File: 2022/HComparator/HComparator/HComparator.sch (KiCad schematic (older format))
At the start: 0 parts

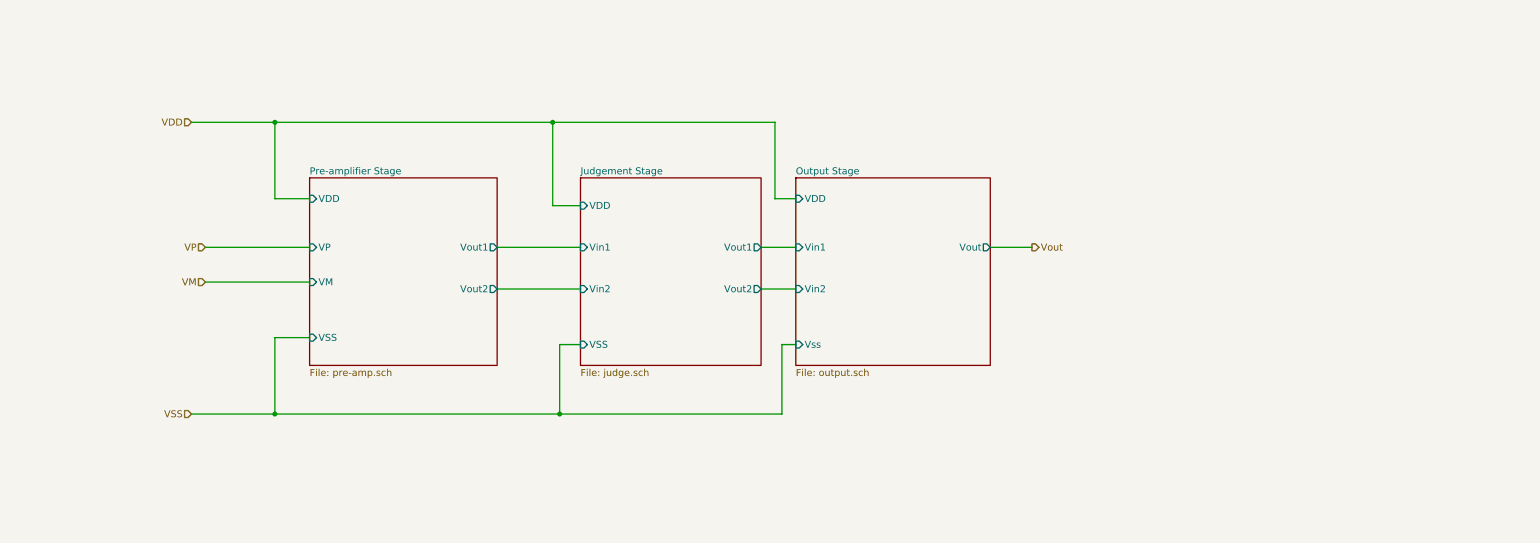
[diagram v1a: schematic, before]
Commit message: へ〜いとにかくセーブ
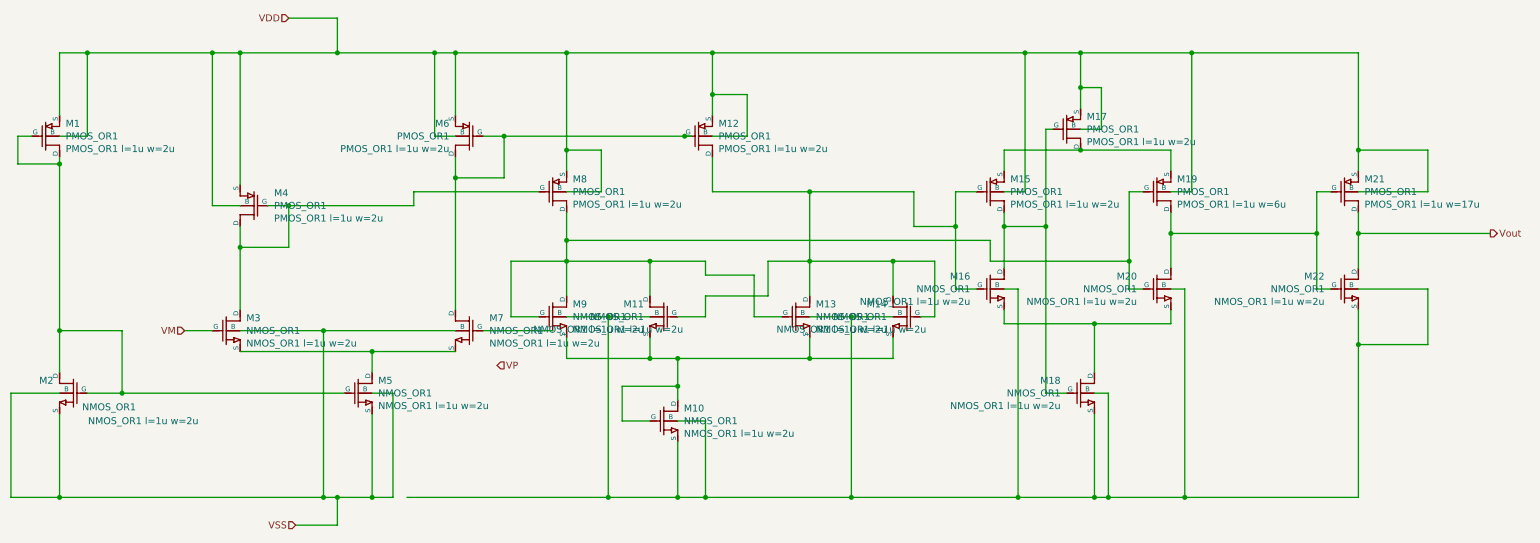
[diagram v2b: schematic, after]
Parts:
- added M1, M12, M15, M17, M19, M21, M4, M6, M8: PMOS_OR1, symbol 0_OR1Symbols:PMOS_OR1
- added M10, M11, M13, M14, M16, M18, M2, M20, M22, M3, M5, M7, M9: NMOS_OR1, symbol 0_OR1Symbols:NMOS_OR1
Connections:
- net VDD: now also M1.3 (S), M1.4 (B), M12.3 (S), M12.4 (B), M15.4 (B), M17.3 (S), M17.4 (B), M19.4 (B), M21.3 (S), M21.4 (B), M4.3 (S), M4.4 (B), M6.3 (S), M6.4 (B), M8.3 (S), M8.4 (B)
- net VM: now also M3.2 (G)
- net VSS: now also M2.3 (S), M2.4 (B), M3.4 (B), M5.3 (S), M5.4 (B), M7.4 (B)
- net Vout: now also M21.1 (D), M22.1 (D)
- new net: M1.1 (D), M1.2 (G), M2.1 (D), M2.2 (G), M5.2 (G)
- new net: M3.3 (S), M5.1 (D), M7.3 (S)
- new net: M12.2 (G), M6.1 (D), M6.2 (G), M7.1 (D)
- new net: M3.1 (D), M4.1 (D), M4.2 (G), M8.2 (G)
- new net: M11.2 (G), M12.1 (D), M13.1 (D), M14.1 (D), M14.2 (G), M15.2 (G), M16.2 (G)
- new net: M10.1 (D), M10.2 (G), M11.3 (S), M13.3 (S), M14.3 (S), M9.3 (S)
- new net: M10.3 (S), M10.4 (B), M11.4 (B), M13.4 (B), M14.4 (B), M16.4 (B), M18.3 (S), M18.4 (B), M20.4 (B), M22.3 (S), M22.4 (B), M9.4 (B)
- new net: M11.1 (D), M13.2 (G), M19.2 (G), M20.2 (G), M8.1 (D), M9.1 (D), M9.2 (G)
- new net: M19.1 (D), M20.1 (D), M21.2 (G), M22.2 (G)
- new net: M16.3 (S), M18.1 (D), M20.3 (S)
- new net: M15.3 (S), M17.1 (D), M19.3 (S)
- new net: M15.1 (D), M16.1 (D), M17.2 (G), M18.2 (G)
